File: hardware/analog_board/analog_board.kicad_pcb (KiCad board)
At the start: 4 copper layers, 330 parts, among them J1 2x5 牛角座, J2 Conn_02x08_Counter_Clockwise, J3 Conn_01x04_Pin, J4 Conn_01x08, J5 CH1, J6 CH1, Q1 MMBT3906, Q2 MMBT3906, U1 GW2A-LV18EQ144, U10 TPS54360DDA, U11 TPS62933, U12 L7805, U13 L7905, U14 TPS7A4701xRGW, U15 TPS7A91, U19 AMS1117, U2 W25Q32JVSS, U3 AD9747BCPZ, U4 OPA695ID, U5 OPA695ID, U6 NE5532, U8 CDCI6214RGER, U9 TPS54360DDA, Y1 ASE-10MHz

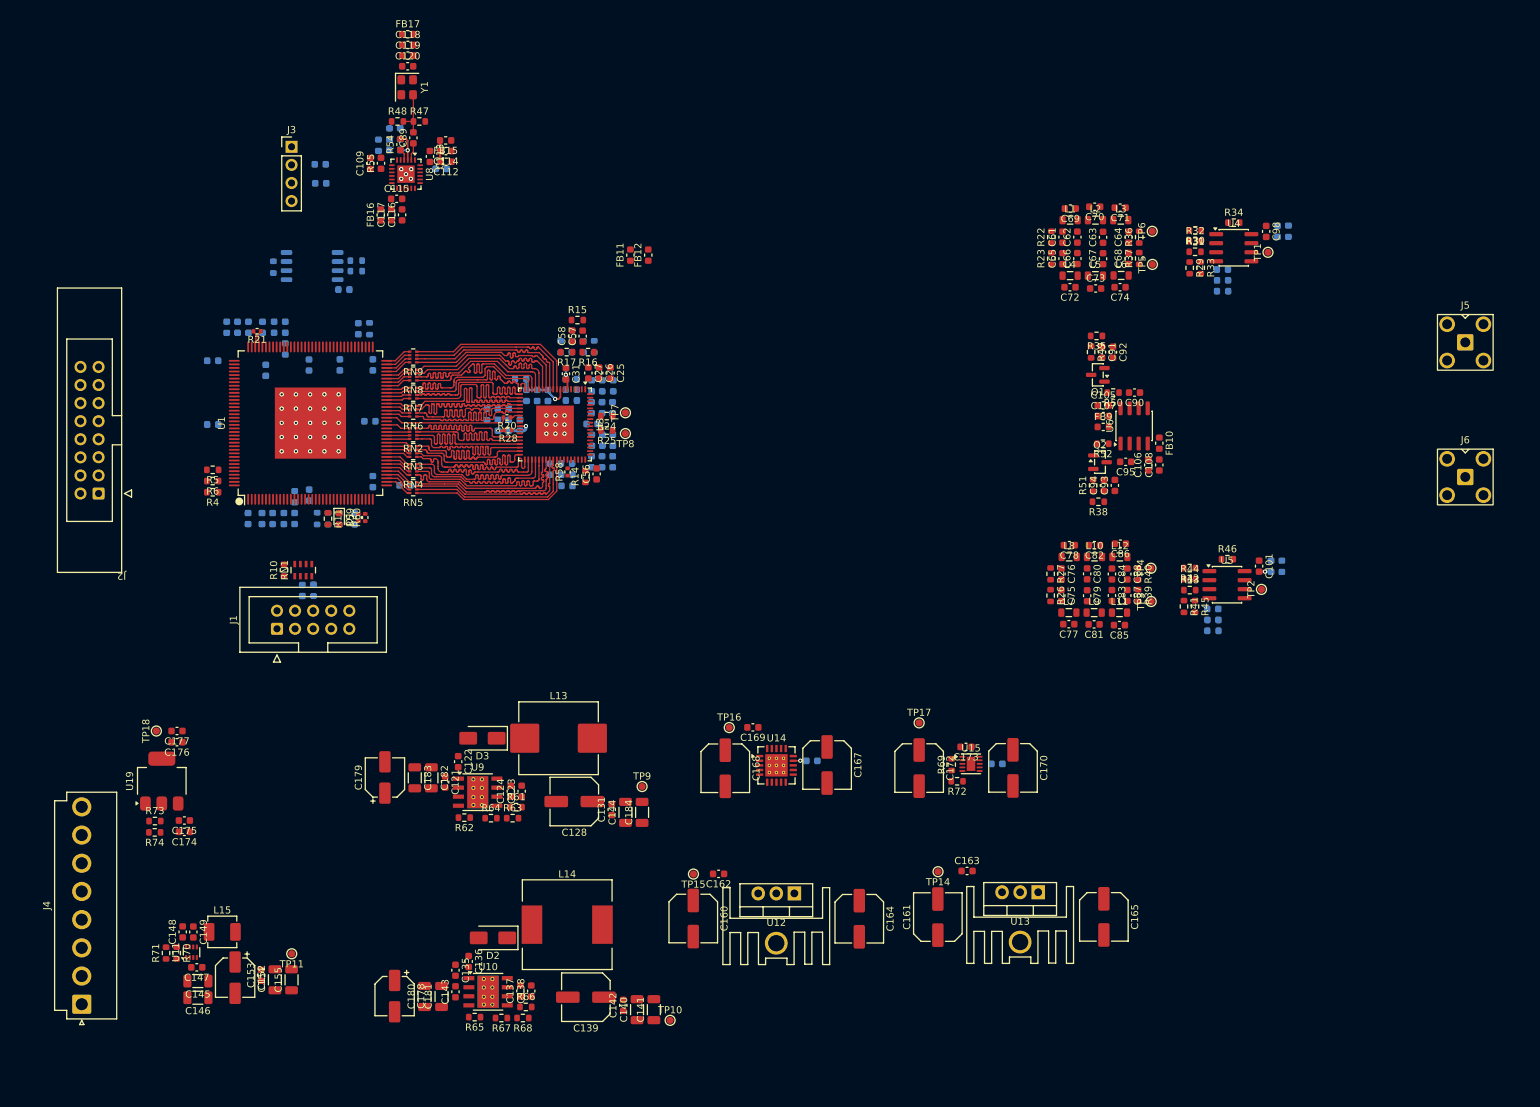
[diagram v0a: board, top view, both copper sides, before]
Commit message: feat：FPGA布线
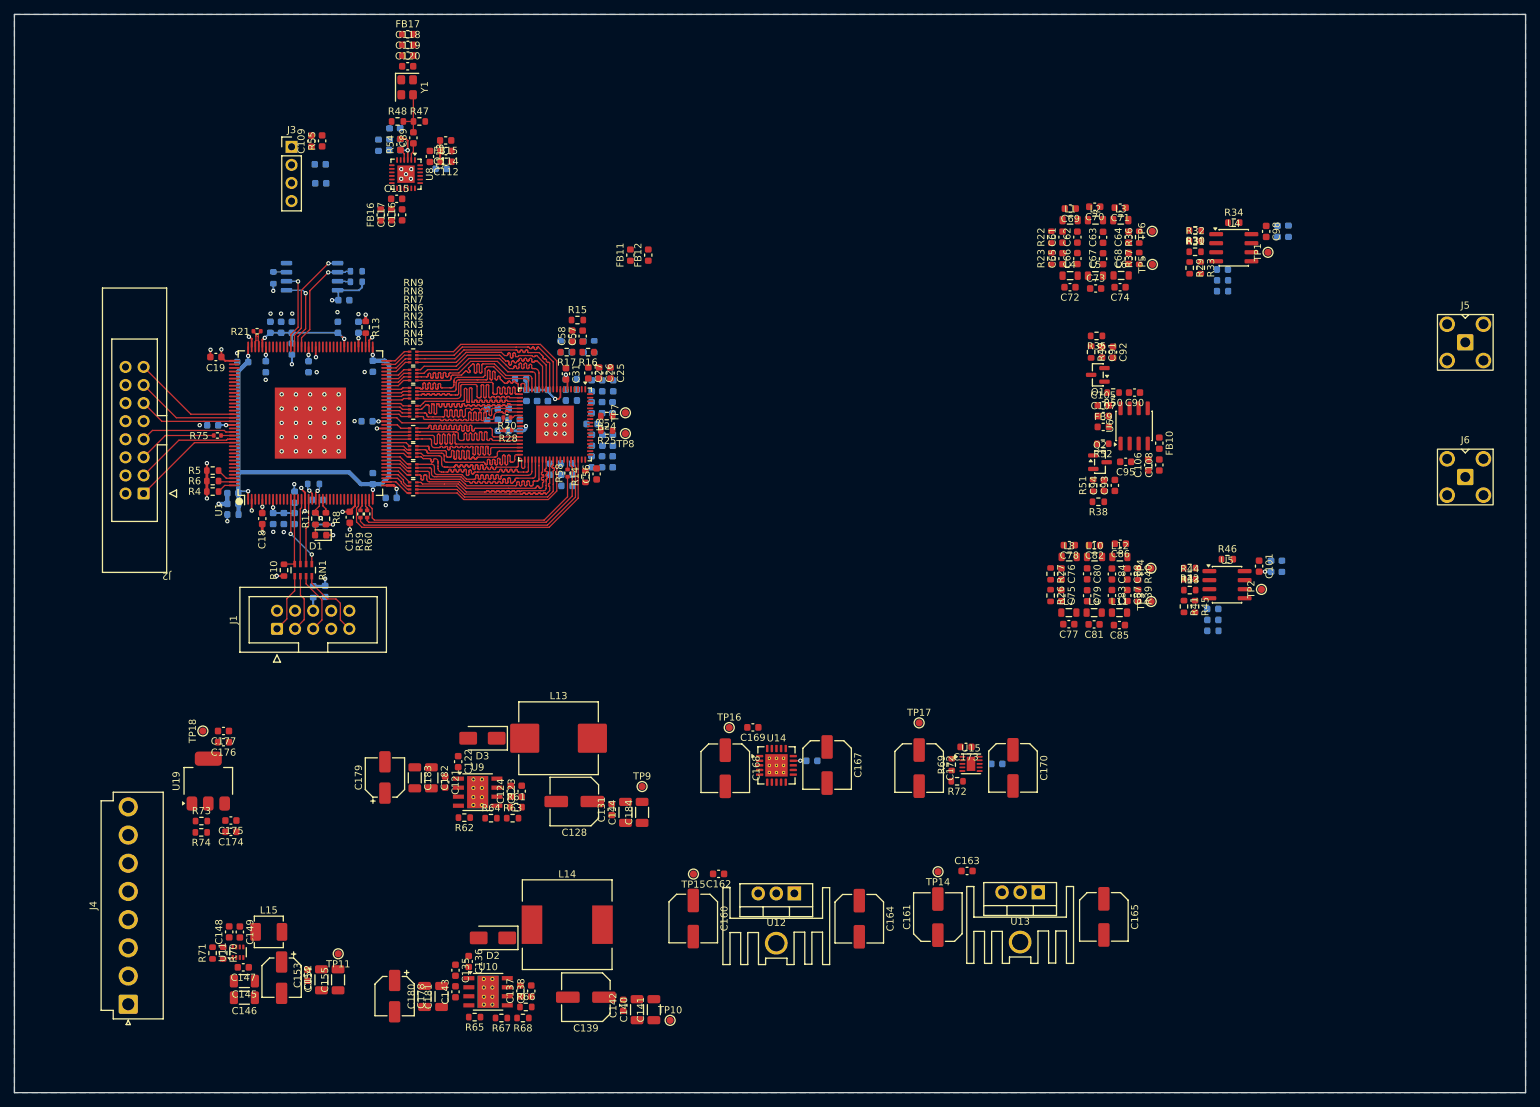
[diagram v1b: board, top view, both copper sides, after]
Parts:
- added R75: 22R, Resistor_SMD:R_0402_1005Metric, F.Cu at (45.0, 71.2)
- C15, C18, C19, R13, R8: moved to F.Cu
- moved FB3 26.3 mm to (47.2, 82.3), turned to 0 degrees
- moved C10 24.8 mm to (47.2, 80.8), turned to 0 degrees
- moved C109 8.85 mm to (58.2, 29.8)
- moved R55 8.85 mm to (59.7, 29.8)
- moved C145 6.53 mm to (48.8, 147.8)
- moved C146 6.53 mm to (48.8, 150.1)
- moved C147 6.53 mm to (48.6, 145.9)
- moved C148 6.53 mm to (46.7, 140.9)
- moved C152 6.53 mm to (54.0, 147.3)
- moved C154 6.53 mm to (59.6, 147.6)
- moved C174 6.53 mm to (46.9, 126.8)
- moved C175 6.53 mm to (46.9, 125.2)
- moved J4 6.53 mm to (32.5, 151.1)
- moved R73 6.53 mm to (42.8, 125.3)
- moved R74 6.53 mm to (42.7, 126.9)
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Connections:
- U1 pad 130: /FPGA_Ctrl.Ctrl_SPI_MISO -> Net-(U1C-IOT17A)
- U14 pad 17: GND -> (no net)
- U14 pad 18: GND -> (no net)
- U14 pad 19: GND -> (no net)
- U14 pad 2: +3.3VA -> (no net)
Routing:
- net VCC_Core: track 0.00 -> 71.3 mm, vias 0 -> 4
- net /DAC/DAC_SPI.DAC_SPI_CS: track 0.00 -> 41.9 mm
- net +3.3V: track 0.00 -> 39.1 mm, vias 0 -> 14
- net /DAC/DAC_SPI.DAC_SPI_CLK: track 0.00 -> 37.9 mm
- net +1V0: track 0.00 -> 37.7 mm, vias 0 -> 3
- net /DAC/DAC_SPI.DAC_SPI_MOSI: track 0.00 -> 36.0 mm
- net /DAC/DAC_SPI.DAC_SPI_MISO: track 0.00 -> 34.5 mm
- net GND: track 6.22 -> 31.0 mm, vias 41 -> 71
- net VCC_PLLR: track 0.00 -> 16.5 mm, vias 0 -> 2
- net /FPGA_Ctrl.Ctrl_SPI_CS: track 0.00 -> 15.7 mm
- net /FPGA_Ctrl.GPIO2: track 0.00 -> 15.5 mm
- net /FPGA_Config/MSPI_MCLK: track 0.00 -> 15.2 mm, vias 0 -> 1
- net /FPGA_Config/MSPI_MO: track 0.00 -> 15.0 mm, vias 0 -> 1
- net /FPGA_Ctrl.Ctrl_SPI_CLK: track 0.00 -> 14.8 mm
- net /FPGA_Ctrl.GPIO1: track 0.00 -> 14.6 mm
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- added copper zone on In2.Cu, net +3.3V
- added copper zone on B.Cu, net GND
- added copper zone on In1.Cu, net GND
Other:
- board outline added: 212.3 x 151.4 mm
